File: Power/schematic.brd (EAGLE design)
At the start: 55 x 60 mm, 10 parts, among them J1 XT60-M, U1 MEZD71203A-F, U2 MEZD71203A-F

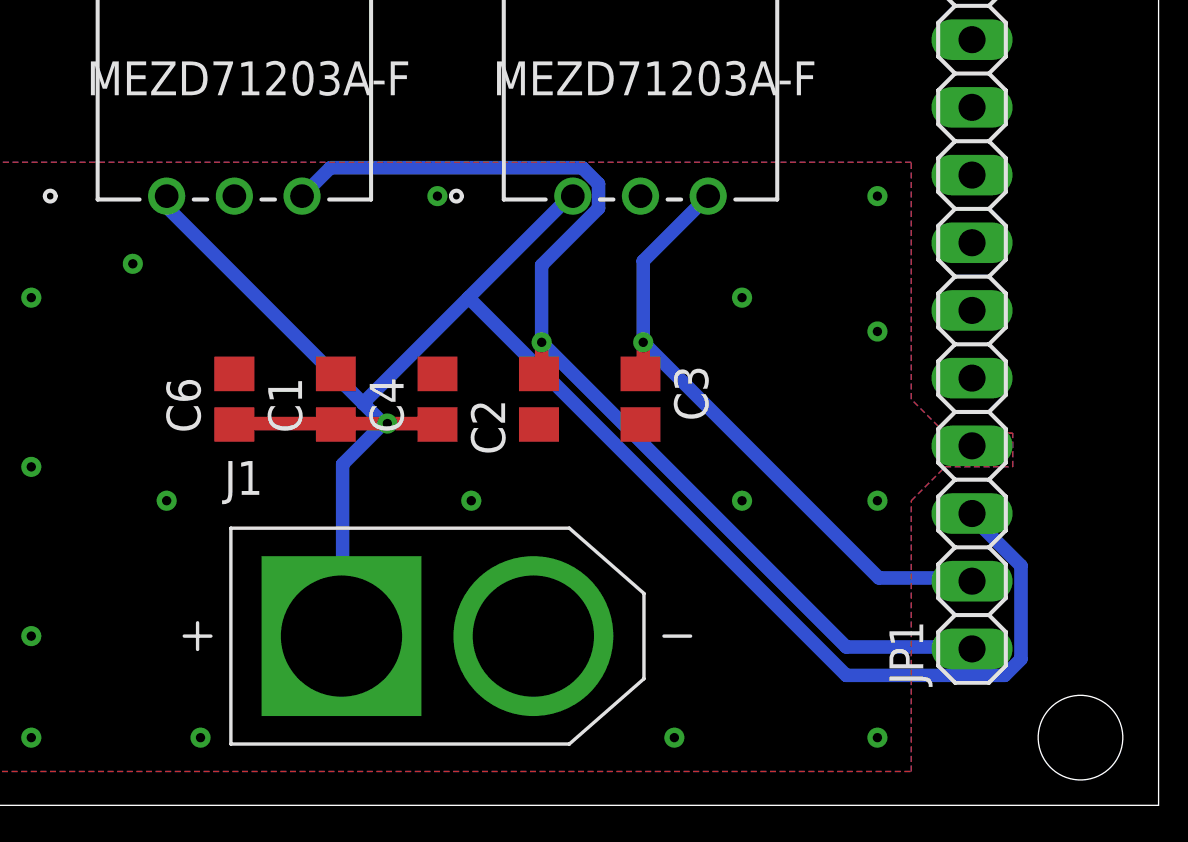
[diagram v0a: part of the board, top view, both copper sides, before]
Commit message: Update schematic.brd
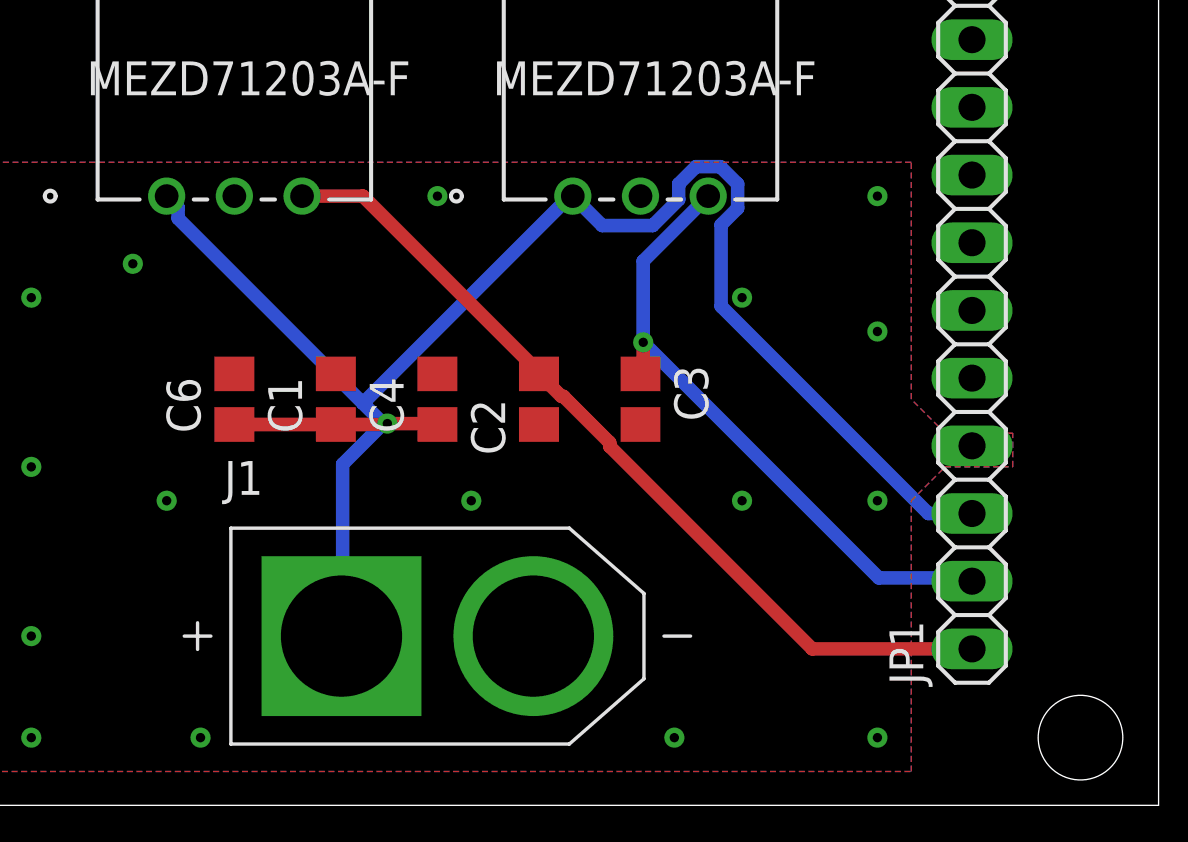
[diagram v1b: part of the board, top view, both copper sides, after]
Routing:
- net 3V3.1: track 41.0 -> 32.3 mm, vias 1 -> 0
- net LIPO: track 73.1 -> 65.3 mm
- net GND: track 4.98 -> 0.00 mm, vias 1 -> 0
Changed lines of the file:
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@@
 <contactref element="U2" pad="2"/>
 <contactref element="C3" pad="2"/>
-<wire x1="31.54" y1="14.08" x2="31.75" y2="14.29" width="0.1524" layer="1"/>
-<wire x1="28.26" y1="16.51" x2="27.94" y2="16.19" width="0.3048" layer="1"/>
-<wire x1="31.75" y1="14.29" x2="32.07795625" y2="13.96204375" width="0.3048" layer="1"/>
-<via x="48" y="13.49" extent="1-16" drill="0.35"/>
-<wire x1="24.45" y1="16.19" x2="24.13" y2="16.51" width="0.3048" layer="1"/>
-<wire x1="24.13" y1="16.19" x2="24.13" y2="16.51" width="0.3048" layer="1"/>
-<wire x1="31.75" y1="14.29" x2="31.75" y2="13.97" width="0.3048" layer="1"/>
-<wire x1="35.56" y1="13.97" x2="35.56" y2="14.29" width="0.3048" layer="1"/>
 <polygon width="0.3048" layer="16">
 <vertex x="10.16" y="1.27"/>
@@
 </polygon>
 <contactref element="C6" pad="2"/>
-<wire x1="32.1564" y1="14.0208" x2="31.75" y2="14.29" width="0.1524" layer="1"/>
-<wire x1="35.5092" y1="14.0208" x2="35.56" y2="14.29" width="0.1524" layer="1"/>
-<wire x1="20.4216" y1="16.1544" x2="20.32" y2="16.19" width="0.1524" layer="1"/>
-<wire x1="24.0792" y1="16.1544" x2="24.13" y2="16.19" width="0.1524" layer="1"/>
-<wire x1="24.5364" y1="16.3068" x2="24.13" y2="16.19" width="0.1524" layer="1"/>
-<wire x1="27.8892" y1="16.3068" x2="27.94" y2="16.19" width="0.1524" layer="1"/>
-<wire x1="31.5468" y1="14.1732" x2="31.75" y2="14.29" width="0.1524" layer="1"/>
-<wire x1="28.3464" y1="16.4592" x2="27.94" y2="16.19" width="0.1524" layer="1"/>
-<wire x1="20.4216" y1="16.3068" x2="20.32" y2="16.19" width="0.1524" layer="1"/>
 <polygon width="0.1524" layer="1">
 <vertex x="10.16" y="24.13"/>
@@
 <contactref element="C6" pad="1"/>
 <wire x1="20.4216" y1="14.3256" x2="20.4216" y2="14.29" width="0.1524" layer="1"/>
-<wire x1="20.2692" y1="14.3256" x2="20.32" y2="14.29" width="0.1524" layer="1"/>
-<wire x1="47.8536" y1="10.9728" x2="48" y2="10.95" width="0.508" layer="16"/>
 <wire x1="33.0708" y1="22.86" x2="33.02" y2="22.86" width="0.508" layer="16"/>
-<wire x1="24.2316" y1="14.1732" x2="24.13" y2="14.29" width="0.1524" layer="1"/>
-<wire x1="24.0792" y1="14.3256" x2="20.4216" y2="14.3256" width="0.508" layer="1"/>
-<wire x1="20.4216" y1="14.3256" x2="20.32" y2="14.29" width="0.1524" layer="1"/>
 <wire x1="24.0792" y1="14.3256" x2="24.13" y2="14.29" width="0.1524" layer="1"/>
 <wire x1="27.8892" y1="14.3256" x2="26.0604" y2="14.3256" width="0.508" layer="1"/>
-<wire x1="26.0604" y1="14.3256" x2="24.2316" y2="14.3256" width="0.508" layer="1"/>
-<wire x1="24.2316" y1="14.3256" x2="24.13" y2="14.29" width="0.1524" layer="1"/>
 <wire x1="27.8892" y1="14.3256" x2="27.94" y2="14.29" width="0.1524" layer="1"/>
 <wire x1="24.384" y1="12.8016" x2="25.908" y2="14.3256" width="0.508" layer="16"/>
 <wire x1="24.384" y1="6.4008" x2="24.384" y2="12.8016" width="0.508" layer="16"/>
 <wire x1="24.384" y1="6.4008" x2="24.34" y2="6.35" width="0.508" layer="16"/>
-<wire x1="17.8308" y1="22.4028" x2="17.8308" y2="22.86" width="0.254" layer="16"/>
 <wire x1="25.908" y1="14.3256" x2="25.146" y2="15.0876" width="0.508" layer="16"/>
-<wire x1="25.146" y1="15.0876" x2="17.8308" y2="22.4028" width="0.508" layer="16"/>
-<wire x1="17.8308" y1="22.86" x2="17.78" y2="22.86" width="0.508" layer="16"/>
+<wire x1="18.2118" y1="22.0218" x2="25.146" y2="15.0876" width="0.508" layer="16"/>
 <wire x1="25.908" y1="14.3256" x2="26.0604" y2="14.3256" width="0.1524" layer="16"/>
-<wire x1="25.146" y1="15.0876" x2="29.1084" y2="19.05" width="0.508" layer="16"/>
-<wire x1="29.1084" y1="19.05" x2="32.9184" y2="22.86" width="0.508" layer="16"/>
+<wire x1="25.146" y1="15.0876" x2="32.9184" y2="22.86" width="0.508" layer="16"/>
 <wire x1="32.9184" y1="22.86" x2="33.02" y2="22.86" width="0.1524" layer="16"/>
-<wire x1="49.8348" y1="8.9916" x2="48.006" y2="10.8204" width="0.508" layer="16"/>
-<wire x1="49.8348" y1="5.4864" x2="49.8348" y2="8.9916" width="0.508" layer="16"/>
-<wire x1="49.2252" y1="4.8768" x2="49.8348" y2="5.4864" width="0.508" layer="16"/>
-<wire x1="43.2816" y1="4.8768" x2="49.2252" y2="4.8768" width="0.508" layer="16"/>
-<wire x1="29.1084" y1="19.05" x2="43.2816" y2="4.8768" width="0.508" layer="16"/>
-<wire x1="48.006" y1="10.8204" x2="48" y2="10.95" width="0.508" layer="16"/>
 <via x="26.0604" y="14.3256" extent="1-16" drill="0.35"/>
+<wire x1="17.78" y1="22.86" x2="18.2118" y2="22.4282" width="0.508" layer="16"/>
+<wire x1="18.2118" y1="22.4282" x2="18.2118" y2="22.0218" width="0.508" layer="16"/>
+<wire x1="36.9951" y1="23.31766875" x2="37.64233125" y2="23.9649" width="0.508" layer="16"/>
+<wire x1="37.64233125" y1="23.9649" x2="38.55766875" y2="23.9649" width="0.508" layer="16"/>
+<wire x1="38.55766875" y1="23.9649" x2="39.2049" y2="23.31766875" width="0.508" layer="16"/>
+<wire x1="39.2049" y1="23.31766875" x2="39.2049" y2="22.40233125" width="0.508" layer="16"/>
+<wire x1="33.02" y1="22.86" x2="34.1249" y2="21.7551" width="0.508" layer="16"/>
+<wire x1="34.1249" y1="21.7551" x2="36.01766875" y2="21.7551" width="0.508" layer="16"/>
+<wire x1="36.01766875" y1="21.7551" x2="36.9951" y2="22.73253125" width="0.508" layer="16"/>
+<wire x1="36.9951" y1="22.73253125" x2="36.9951" y2="23.31766875" width="0.508" layer="16"/>
+<wire x1="46.36040625" y1="10.95" x2="48" y2="10.95" width="0.508" layer="16"/>
+<wire x1="39.2049" y1="22.40233125" x2="38.5854" y2="21.78283125" width="0.508" layer="16"/>
+<wire x1="38.5854" y1="21.78283125" x2="38.5854" y2="18.72500625" width="0.508" layer="16"/>
+<wire x1="38.5854" y1="18.72500625" x2="46.36040625" y2="10.95" width="0.508" layer="16"/>
+<wire x1="20.32" y1="14.29" x2="24.13" y2="14.29" width="0.508" layer="1"/>
+<wire x1="24.13" y1="14.29" x2="26.0248" y2="14.29" width="0.508" layer="1"/>
+<wire x1="26.0248" y1="14.29" x2="26.0604" y2="14.3256" width="0.508" layer="1"/>
 </signal>
 <signal name="SCL0">
@@
 <contactref element="JP1" pad="1"/>
 <wire x1="31.6992" y1="16.3068" x2="31.75" y2="16.19" width="0.1524" layer="1"/>
-<wire x1="31.8516" y1="16.1544" x2="31.75" y2="16.19" width="0.1524" layer="1"/>
-<wire x1="31.8516" y1="17.3736" x2="31.8516" y2="16.3068" width="0.508" layer="1"/>
-<wire x1="31.8516" y1="20.2692" x2="31.8516" y2="17.3736" width="0.508" layer="16"/>
-<wire x1="33.9852" y1="22.4028" x2="31.8516" y2="20.2692" width="0.508" layer="16"/>
-<wire x1="33.9852" y1="23.3172" x2="33.9852" y2="22.4028" width="0.508" layer="16"/>
-<wire x1="33.3756" y1="23.9268" x2="33.9852" y2="23.3172" width="0.508" layer="16"/>
-<wire x1="23.9268" y1="23.9268" x2="33.3756" y2="23.9268" width="0.508" layer="16"/>
-<wire x1="22.86" y1="22.86" x2="23.9268" y2="23.9268" width="0.508" layer="16"/>
-<wire x1="31.8516" y1="16.3068" x2="31.75" y2="16.19" width="0.1524" layer="1"/>
-<wire x1="43.2816" y1="5.9436" x2="47.8536" y2="5.9436" width="0.508" layer="16"/>
-<wire x1="31.8516" y1="17.3736" x2="43.2816" y2="5.9436" width="0.508" layer="16"/>
-<wire x1="47.8536" y1="5.9436" x2="48" y2="5.87" width="0.508" layer="16"/>
-<via x="31.8516" y="17.3736" extent="1-16" drill="0.35"/>
+<wire x1="22.86" y1="22.86" x2="25.146" y2="22.86" width="0.508" layer="1"/>
+<wire x1="25.146" y1="22.86" x2="31.6992" y2="16.3068" width="0.508" layer="1"/>
+<wire x1="31.75" y1="16.19" x2="32.5936" y2="15.3464" width="0.508" layer="1"/>
+<wire x1="32.5936" y1="15.3464" x2="32.6683375" y2="15.3464" width="0.508" layer="1"/>
+<wire x1="32.6683375" y1="15.3464" x2="34.4036" y2="13.6111375" width="0.508" layer="1"/>
+<wire x1="34.4036" y1="13.6111375" x2="34.4036" y2="13.4716625" width="0.508" layer="1"/>
+<wire x1="34.4036" y1="13.4716625" x2="42.0052625" y2="5.87" width="0.508" layer="1"/>
+<wire x1="42.0052625" y1="5.87" x2="48" y2="5.87" width="0.508" layer="1"/>
 </signal>
 <signal name="3V3.2">
